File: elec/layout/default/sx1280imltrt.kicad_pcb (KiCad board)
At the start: 2 copper layers, 225.7 x 100.8 mm, 0 parts

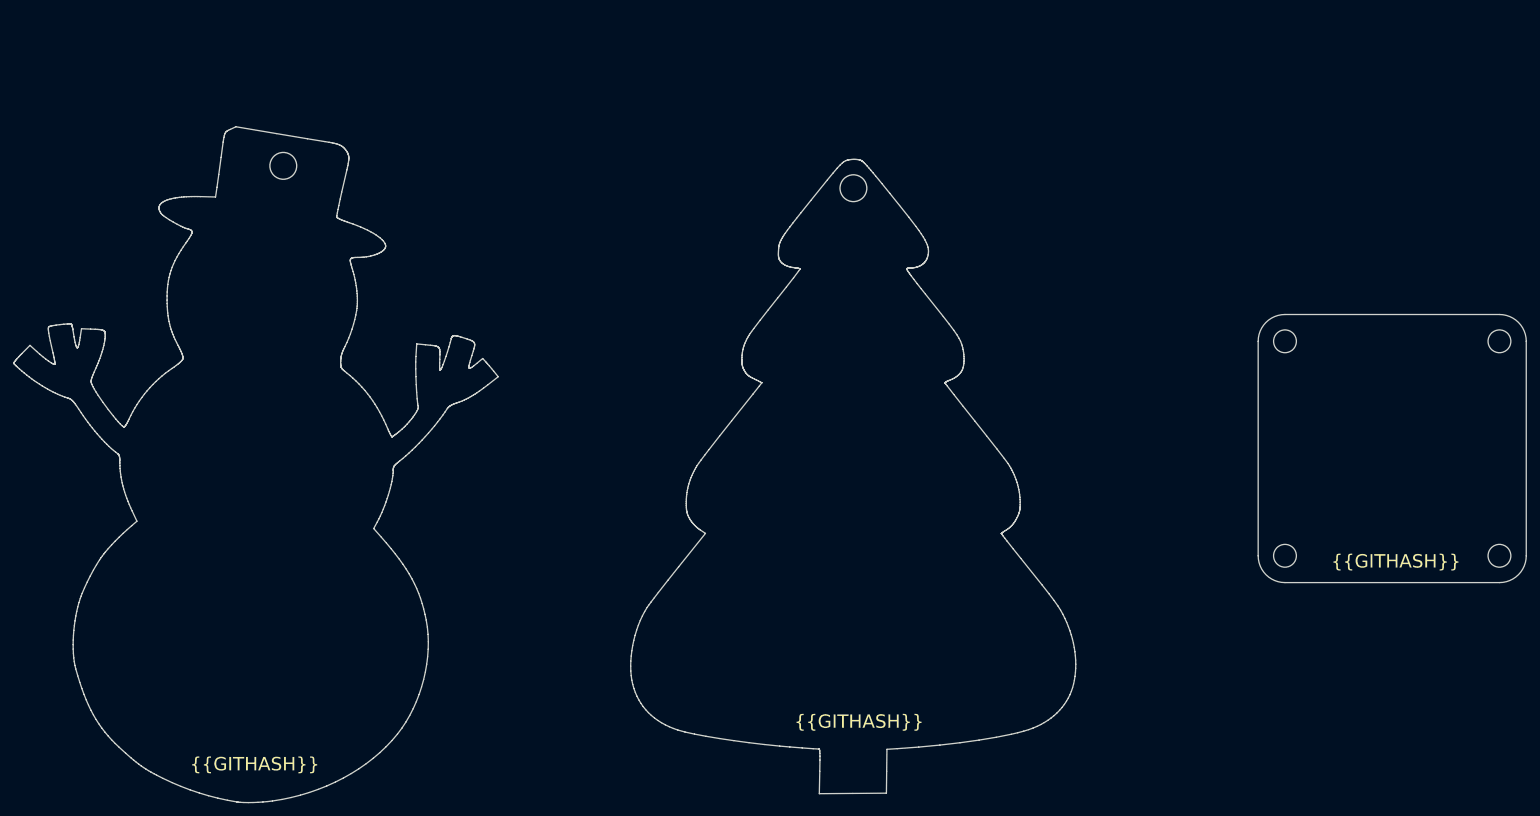
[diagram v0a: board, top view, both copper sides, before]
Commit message: layout
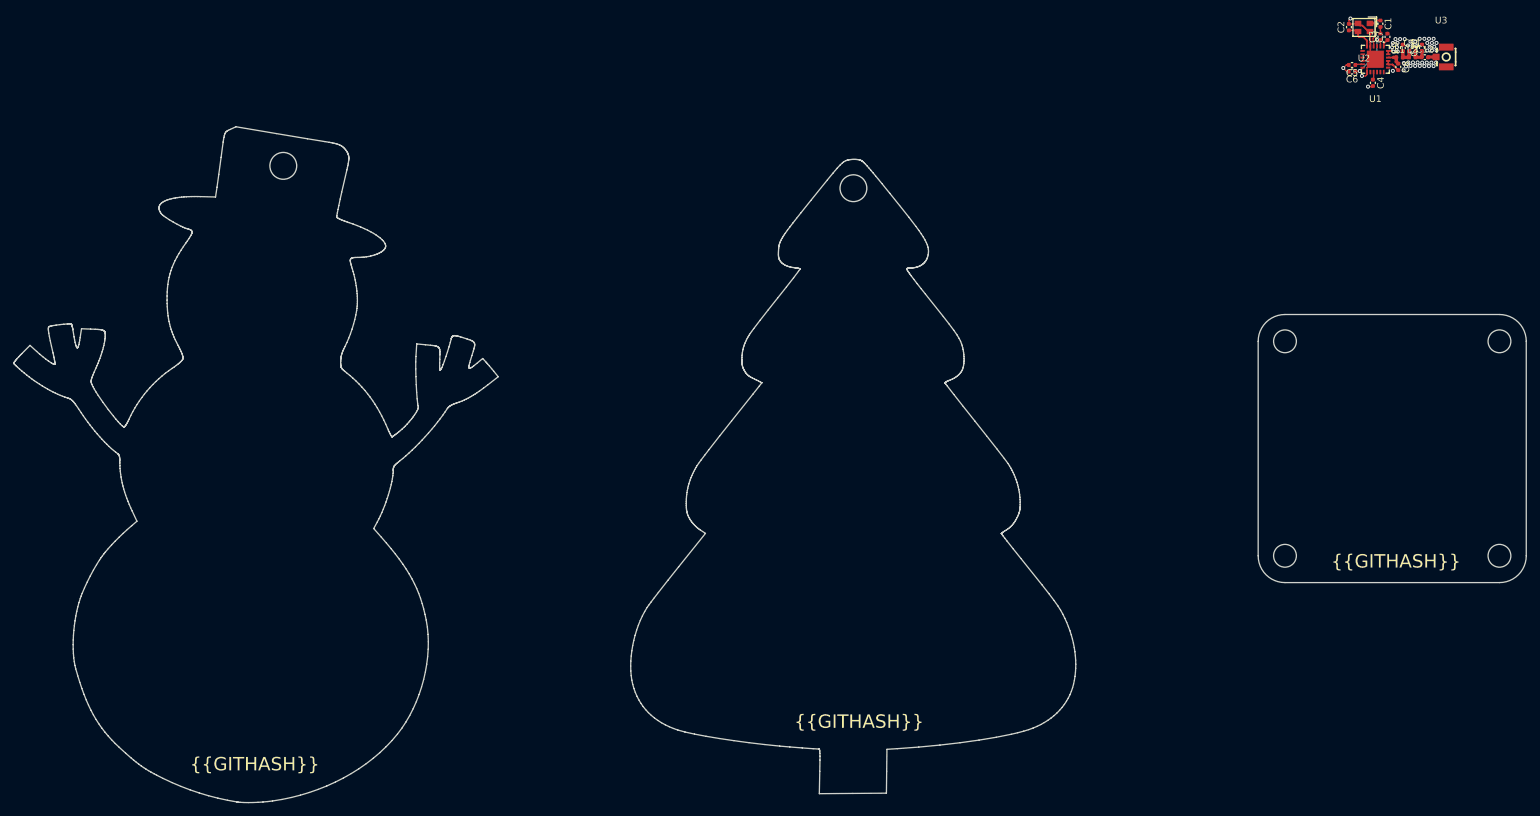
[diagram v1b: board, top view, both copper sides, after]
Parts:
- added C1: 50V 11pF C0G ±5% 0402 Multilayer Ceramic Capacitors MLCC - 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, lib:C0402, F.Cu at (239.9, 34.4)
- added C10: 50V 1pF C0G 0402 Multilayer Ceramic Capacitors MLCC - SMD/S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, lib:C0402, F.Cu at (246.1, 38.0)
- added C11: 50V 1pF C0G 0402 Multilayer Ceramic Capacitors MLCC - SMD/S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, lib:C0402, F.Cu at (244.6, 38.4)
- added C12: 50V 100pF C0G ±5% 0402 Multilayer Ceramic Capacitors MLCC -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, lib:C0402, F.Cu at (246.5, 39.4)
- added C2: 50V 11pF C0G ±5% 0402 Multilayer Ceramic Capacitors MLCC - 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, lib:C0402, F.Cu at (235.2, 34.9)
- added C3: 10V 470nF X5R ±10% 0402 Multilayer Ceramic Capacitors MLCC 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, lib:C0402, F.Cu at (239.9, 36.4)
- added C4: Multilayer Ceramic Capacitors MLCC - SMD/SMT 100nF 10V 0402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, lib:C0402, F.Cu at (238.7, 43.2)
- added C5: Multilayer Ceramic Capacitors MLCC - SMD/SMT 100nF 10V 0402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, lib:C0402, F.Cu at (235.6, 40.6)
- added C6: 50V 10nF X7R ±10% 0402 Multilayer Ceramic Capacitors MLCC -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, lib:C0402, F.Cu at (235.6, 41.5)
- added C7: 50V 10nF X7R ±10% 0402 Multilayer Ceramic Capacitors MLCC -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, lib:C0402, F.Cu at (240.9, 36.4)
- added C8: 50V 1pF C0G 0402 Multilayer Ceramic Capacitors MLCC - SMD/S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, lib:C0402, F.Cu at (242.5, 40.8)
- added C9: 50V 1pF C0G 0402 Multilayer Ceramic Capacitors MLCC - SMD/S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, lib:C0402, F.Cu at (243.2, 38.0)
- added L1: , lib:L0402, F.Cu at (242.7, 39.4)
- added L2: , lib:L0402, F.Cu at (244.6, 39.4)
- added U1: , lib:QFN-24_L4.0-W4.0-P0.50-BL-EP2.6, F.Cu at (239.1, 39.7)
- added U2: , lib:OSC-SMD_4P-L2.0-W1.6-BL, F.Cu at (237.4, 35.0)
- added U3: , lib:IPEX-SMD_BWIPX-1-001E, F.Cu at (248.9, 39.4)
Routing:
- net gnd: track 0.00 -> 21.7 mm, vias 0 -> 47
- net vcc-1: track 0.00 -> 8.78 mm, vias 0 -> 2
- net xta: track 0.00 -> 6.08 mm
- net xtb: track 0.00 -> 4.74 mm
- net vcc-5: track 0.00 -> 2.86 mm
- net vcc-4: track 0.00 -> 2.86 mm
- net vcc-2: track 0.00 -> 2.31 mm
- net io: track 0.00 -> 2.28 mm
- net gnd-3: track 0.00 -> 1.21 mm
- net vcc: track 0.00 -> 1.18 mm
